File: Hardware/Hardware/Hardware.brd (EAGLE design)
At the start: 58.4 x 63.4 mm, 12 parts, among them J1 1x10 HEADER "A", J2 1x10 HEADER "B", U1 MAX3232

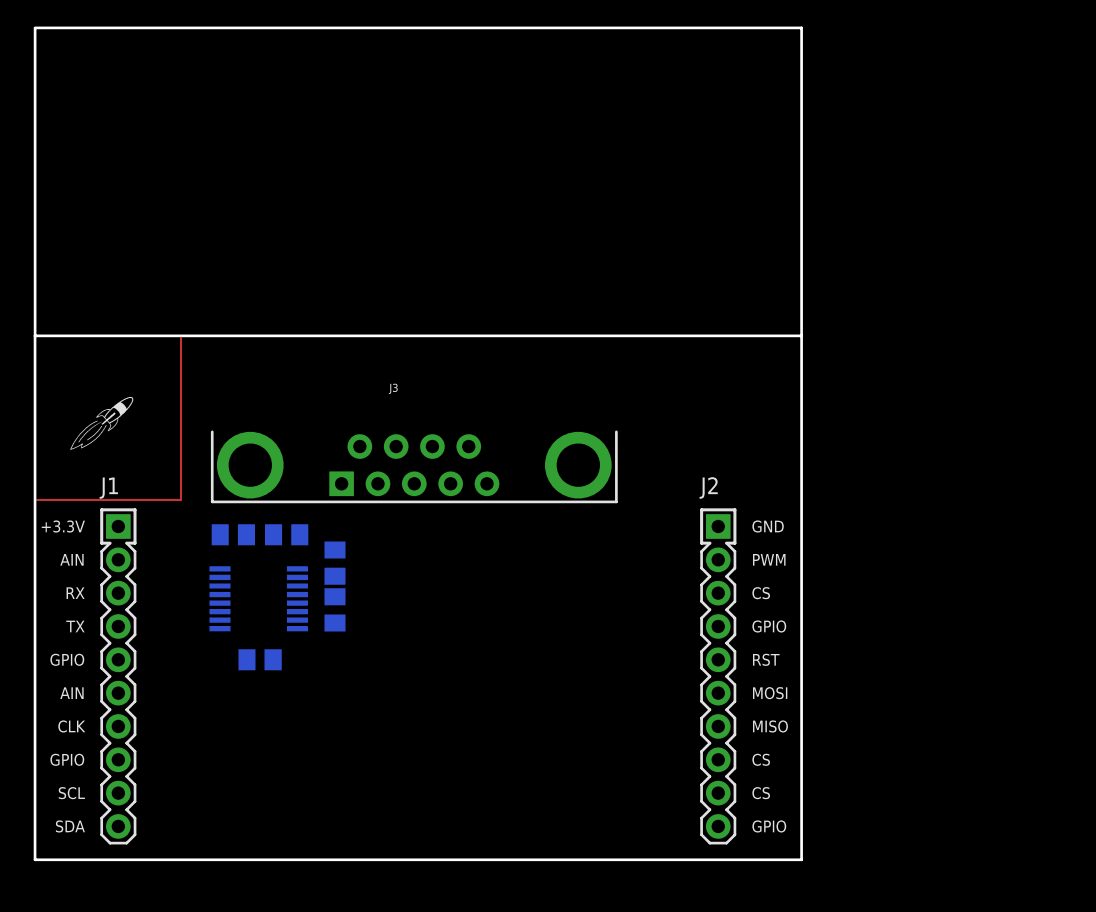
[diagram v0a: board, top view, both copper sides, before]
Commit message: Merged and tidied up the circuit, did my part of PCB
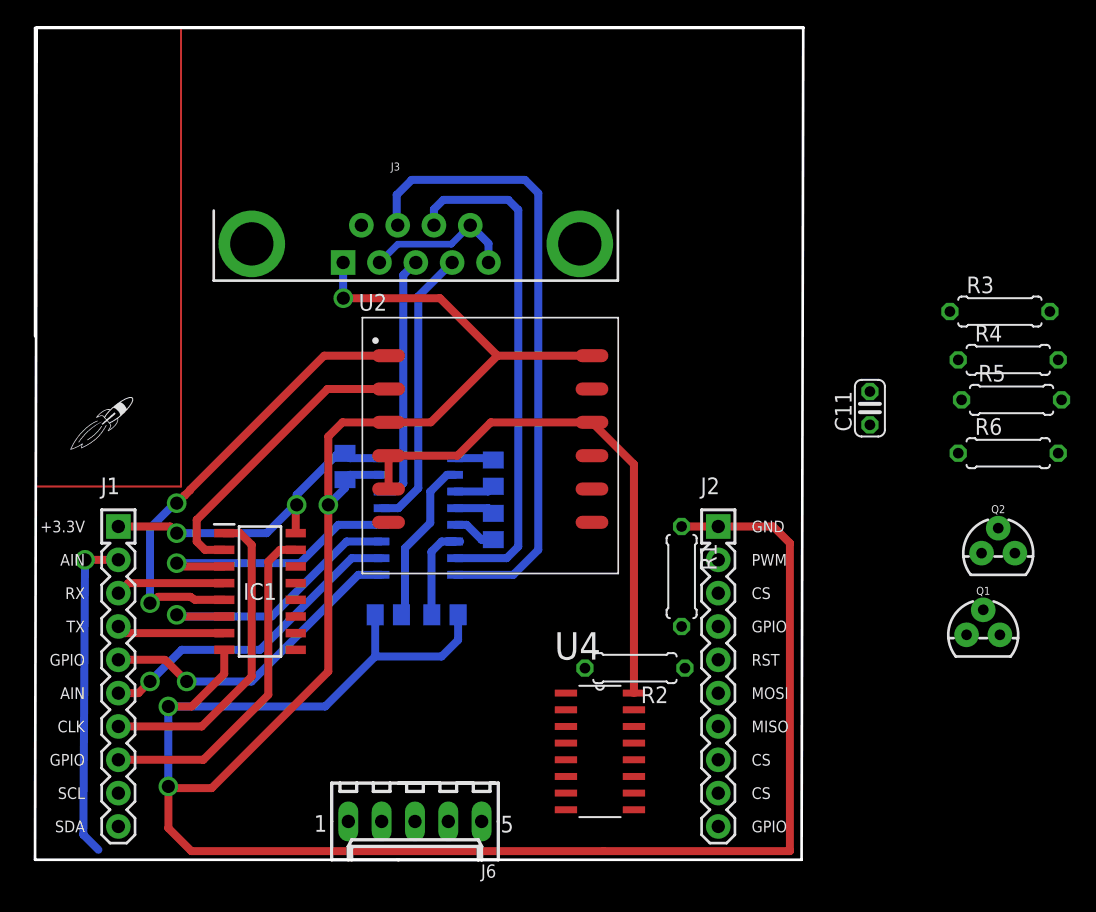
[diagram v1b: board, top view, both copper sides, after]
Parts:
- added C11: 1uF, rcl:C025-024X044
- added IC1: 74FST3257DR2G, 74FST3257DR2G:SOIC127P600X175-16N
- added J6: 22-27-2051-05, con-molex:6410-05
- added Q1, Q2: 200mA/40V, SparkFun-DiscreteSemi:TO-92
- added R1, R2: (no value), rcl:0207/7
- added R3, R6: 1K, rcl:0207/7
- added R4, R5: 4.7K, rcl:0207/7
- added U2: L86-M33, L86-M33:SON254P1840X1840X40-12N
- added U4: 74HC4051D,652, 74HC4051D_652:SOIC127P600X175-16N
- U1: device SparkFun-IC-Comms:TSSOP16 -> SparkFun-IC-Comms:SO16
- moved J3 16.9 mm to (29.0, 46.9)
- moved C4 14.5 mm to (31.2, 18.7), turned to 0 degrees
- moved C1 13.9 mm to (34.9, 29.5)
- moved C2 13.6 mm to (34.9, 25.4)
- moved U1 13.6 mm to (29.2, 26.2)
- moved C5 9.98 mm to (23.6, 30.0), turned to 90 degrees
- moved C3 9.86 mm to (26.9, 18.7)
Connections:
- removed net N$9 (its old number): J1.4, U1.11
- new net +3V3: C5.2, IC1.16, J1.1, Q1.3, R3.2, U1.16, U2.10, U2.4, U2.5, U4.16
- new net N$10: IC1.5, U2.1
- new net N$11: IC1.3, U1.12
- new net N$17: IC1.6, U1.11
- new net N$18: IC1.1, J1.7
- new net N$19: IC1.15, J1.8
- new net N$20: J6.3, U4.13
- new net N$22: J6.2, U4.14
- new net N$23: J6.1, U4.15
- new net N$24: J6.4, U4.12
- new net N$25: R2.2, U4.3
- new net N$3: IC1.4, J1.3
- new net N$47: J1.2, R1.2, R2.1
- new net N$49: J2.8, U4.11
- new net N$50: J2.9, U4.10
- new net N$51: J2.10, U4.9
- new net N$52: C11.2, R4.1, R5.1
- new net N$53: C11.1, J2.2
- new net N$54: Q2.2, R5.2, R6.1
- new net N$55: Q1.2, R3.1, R4.2
- new net N$57: Q1.1, Q2.3
- net GND: now also IC1.8, J2.1, J6.5, Q2.1, R1.1, R6.2, U2.12, U2.3, U4.6, U4.7, U4.8
- net N$5: now also IC1.7, J1.4; no longer C5.2, J1.1, U1.16
- net N$8: now also IC1.2, U2.2; no longer J1.3, U1.12
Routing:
- net GND: track 0.00 -> 204.1 mm, vias 0 -> 4
- net +3V3: track 0.00 -> 66.6 mm, vias 0 -> 2
- net N$15: track 0.00 -> 48.3 mm
- net N$16: track 0.00 -> 39.1 mm
- net N$10: track 0.00 -> 35.3 mm, vias 0 -> 2
- net N$19: track 0.00 -> 26.1 mm
- net N$47: track 0.00 -> 25.1 mm, vias 0 -> 1
- net N$21: track 0.00 -> 24.3 mm, vias 0 -> 1
- net N$18: track 0.00 -> 24.2 mm
- net N$43: track 0.00 -> 24.1 mm, vias 0 -> 1
- net N$8: track 0.00 -> 22.8 mm
- net CUT: track 23.5 -> 45.9 mm
- net N$17: track 0.00 -> 21.7 mm, vias 0 -> 1
- net N$13: track 0.00 -> 21.7 mm
- net N$11: track 0.00 -> 20.6 mm, vias 0 -> 1
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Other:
- board size 58.4 x 63.4 mm -> 58.5 x 63.4 mm
